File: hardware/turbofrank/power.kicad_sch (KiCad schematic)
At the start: 8 parts, among them J3 USB4215, U1 NCP1117 3.3

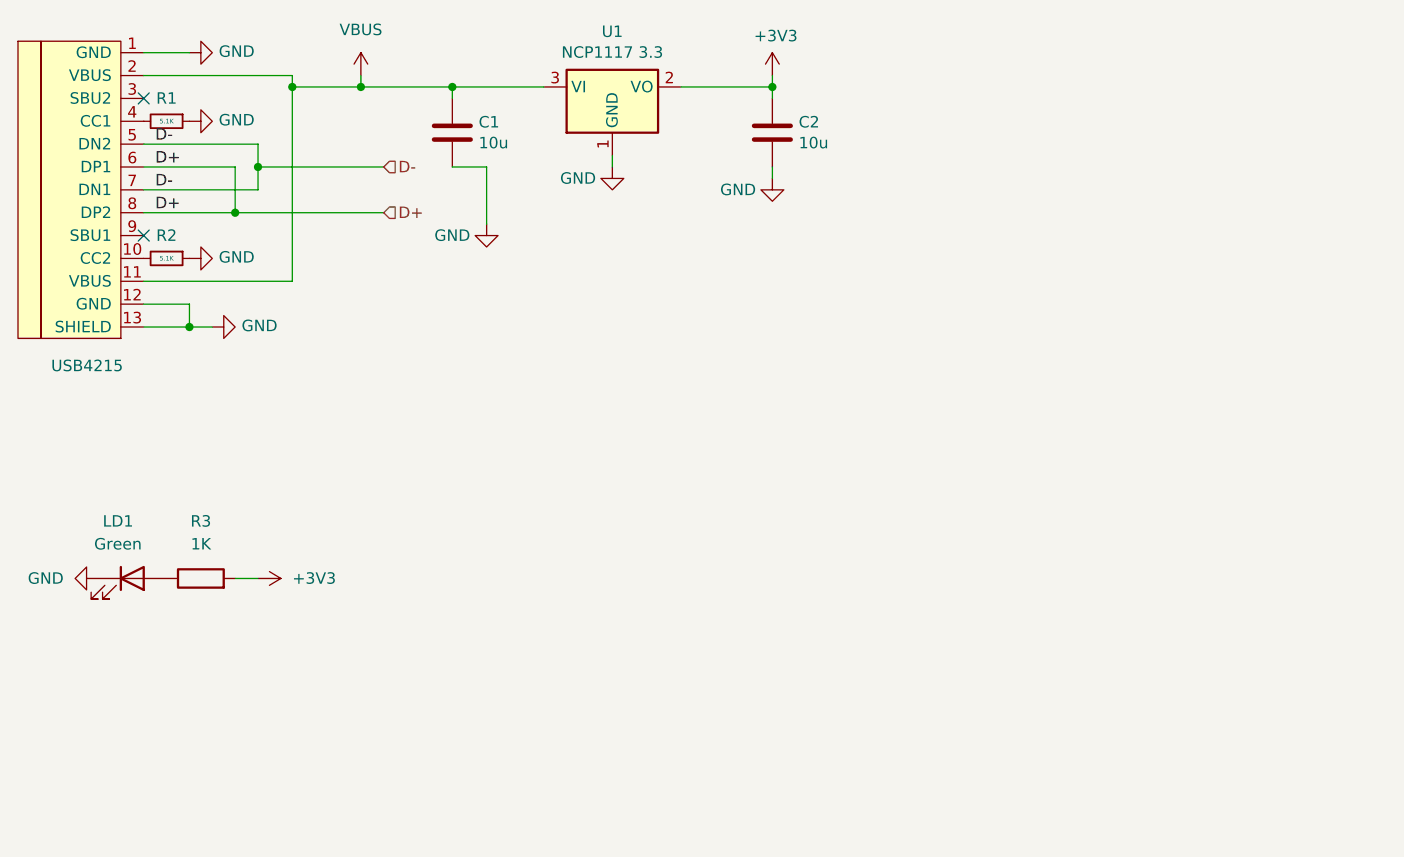
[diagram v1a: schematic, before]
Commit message: TurboFRANK WIP
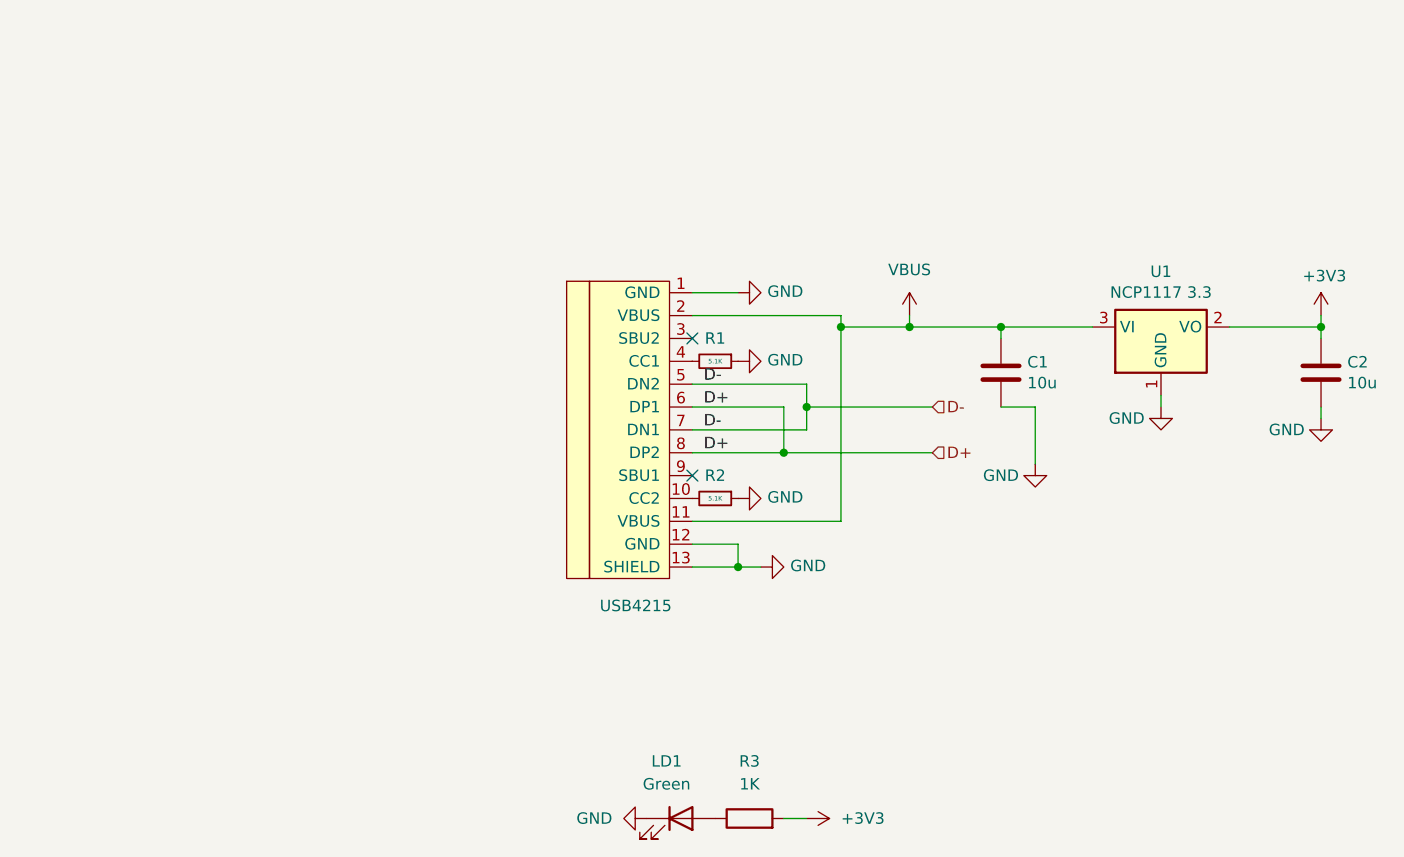
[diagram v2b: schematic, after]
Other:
- moved on the sheet: C1, C2, LD1, R1, R2, R3, U1

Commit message: Bugfixes
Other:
- title: TurboFRANK -> ${NAME}
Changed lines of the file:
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@@
 	(paper "A4")
 	(title_block
-		(title "TurboFRANK")
-		(date "2025-04-04")
+		(title "${NAME}")
+		(date "2025-04-20")
 		(rev "${VERSION}")
 		(company "Mikhail Matveev")
